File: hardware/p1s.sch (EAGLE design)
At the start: 32 parts, among them IC1 74LS595N, IC2 74ALS04N, IC3 74ALS04N, J0 DC24V, Q1 60V/32A/35mΩ, Q2 60V/32A/35mΩ, Q3 60V/32A/35mΩ, Q4 60V/32A/35mΩ, Q5 60V/32A/35mΩ, Q6 60V/32A/35mΩ, Q7 60V/32A/35mΩ, Q8 60V/32A/35mΩ

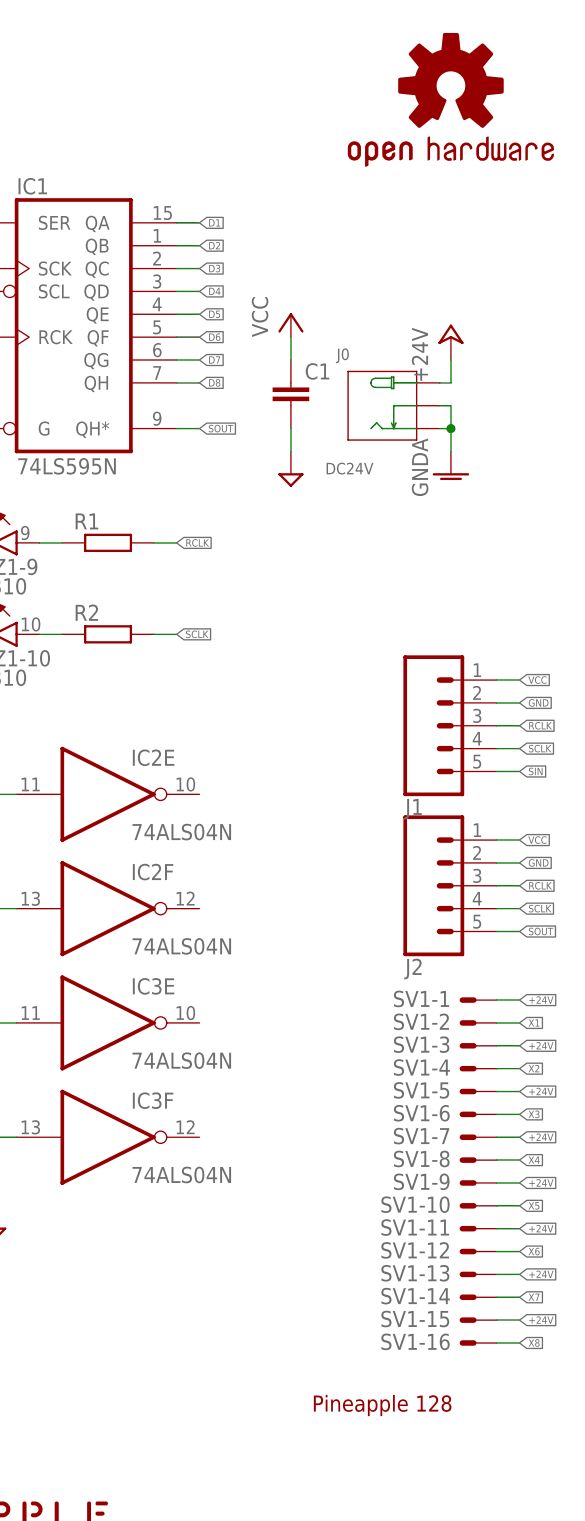
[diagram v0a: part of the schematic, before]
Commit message: Updated P1S.
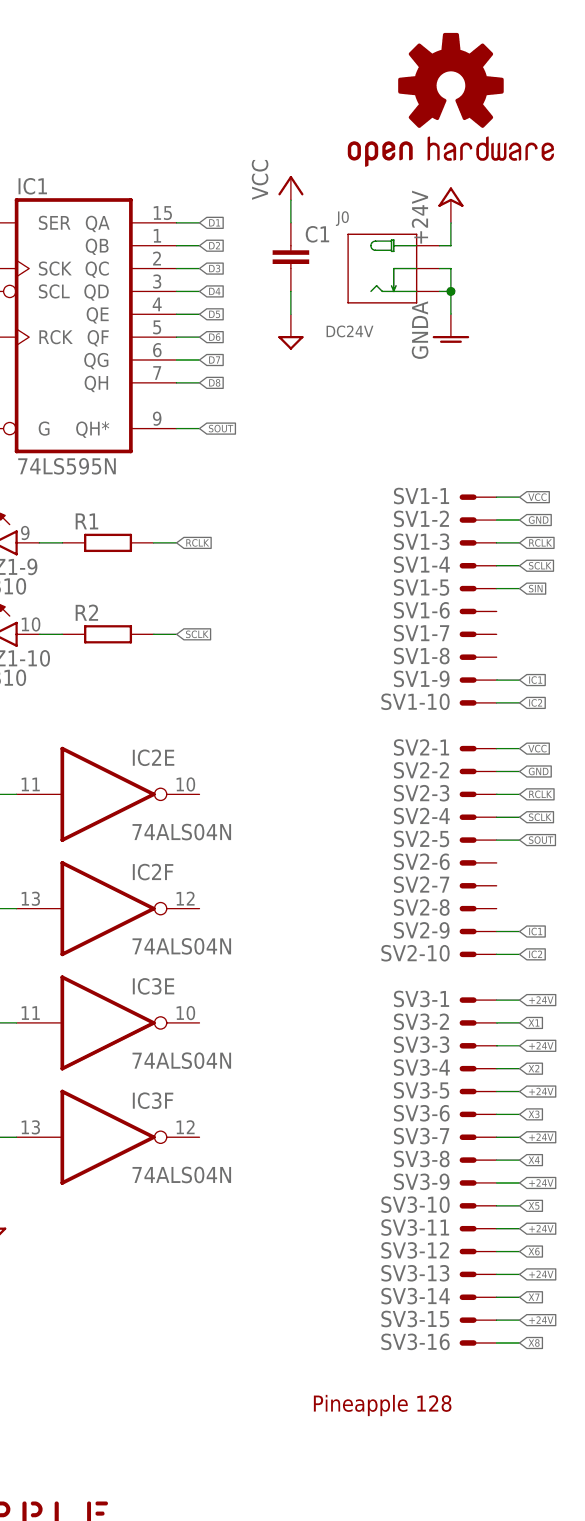
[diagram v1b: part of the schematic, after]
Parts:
- removed J1, J2: (no value), SparkFun-Connectors:CONN_05JST
- added SV2: (no value), con-ml:ML10LE
- added SV3: (no value), con-ml:ML16LE
- SV1: device con-ml:ML16LE -> con-ml:ML10LE
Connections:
- new net IC1: SV1-9.S, SV2-9.S
- new net IC2: SV1-10.S, SV2-10.S
- net +24V: now also SV3-1.S, SV3-11.S, SV3-13.S, SV3-15.S, SV3-3.S, SV3-5.S, SV3-7.S, SV3-9.S; no longer SV1-1.S, SV1-11.S, SV1-13.S, SV1-15.S, SV1-3.S, SV1-5.S, SV1-7.S, SV1-9.S
- net GND: now also SV1-2.S, SV2-2.S; no longer J1.2, J2.2
- net RCLK: now also SV1-3.S, SV2-3.S; no longer J1.3, J2.3
- net SCLK: now also SV1-4.S, SV2-4.S; no longer J1.4, J2.4
- net SIN: now also SV1-5.S; no longer J1.5
- net SOUT: now also SV2-5.S; no longer J2.5
- net VCC: now also SV1-1.S, SV2-1.S; no longer J1.1, J2.1
- net X1: now also SV3-2.S; no longer SV1-2.S
- net X2: now also SV3-4.S; no longer SV1-4.S
- net X3: now also SV3-6.S; no longer SV1-6.S
- net X4: now also SV3-8.S; no longer SV1-8.S
- net X5: now also SV3-10.S; no longer SV1-10.S
- net X6: now also SV3-12.S; no longer SV1-12.S
- net X7: now also SV3-14.S; no longer SV1-14.S
- net X8: now also SV3-16.S; no longer SV1-16.S
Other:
- moved on the sheet: C1, J0, SV1-1, SV1-10, SV1-2, SV1-3, SV1-4, SV1-5, SV1-6, SV1-7, SV1-8, SV1-9
